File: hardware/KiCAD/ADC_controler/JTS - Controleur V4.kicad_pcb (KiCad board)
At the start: 2 copper layers, 119 x 114 mm, 26 parts, among them J1 Power in, J5 Power out, Q1 Q_NMOS_DGS, Q2 Q_NMOS_DGS, Q3 Q_NMOS_DGS, U1 AD797

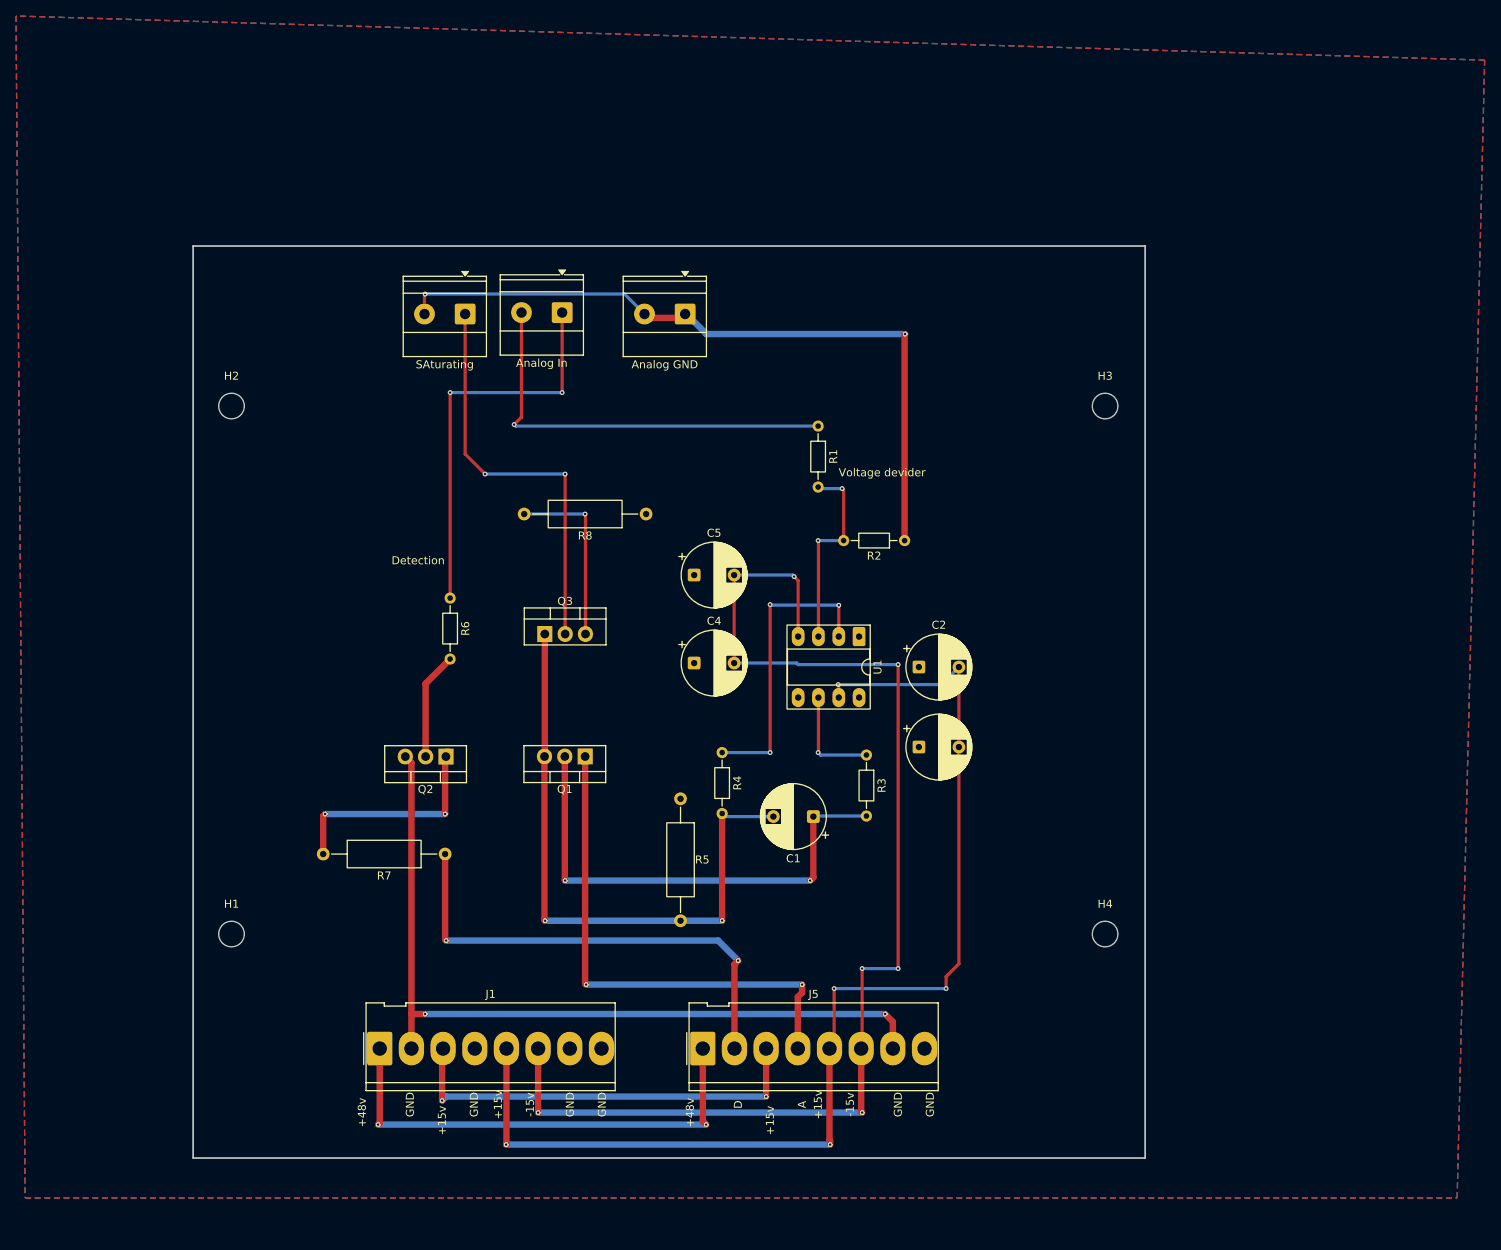
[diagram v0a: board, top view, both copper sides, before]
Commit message: new kicad files
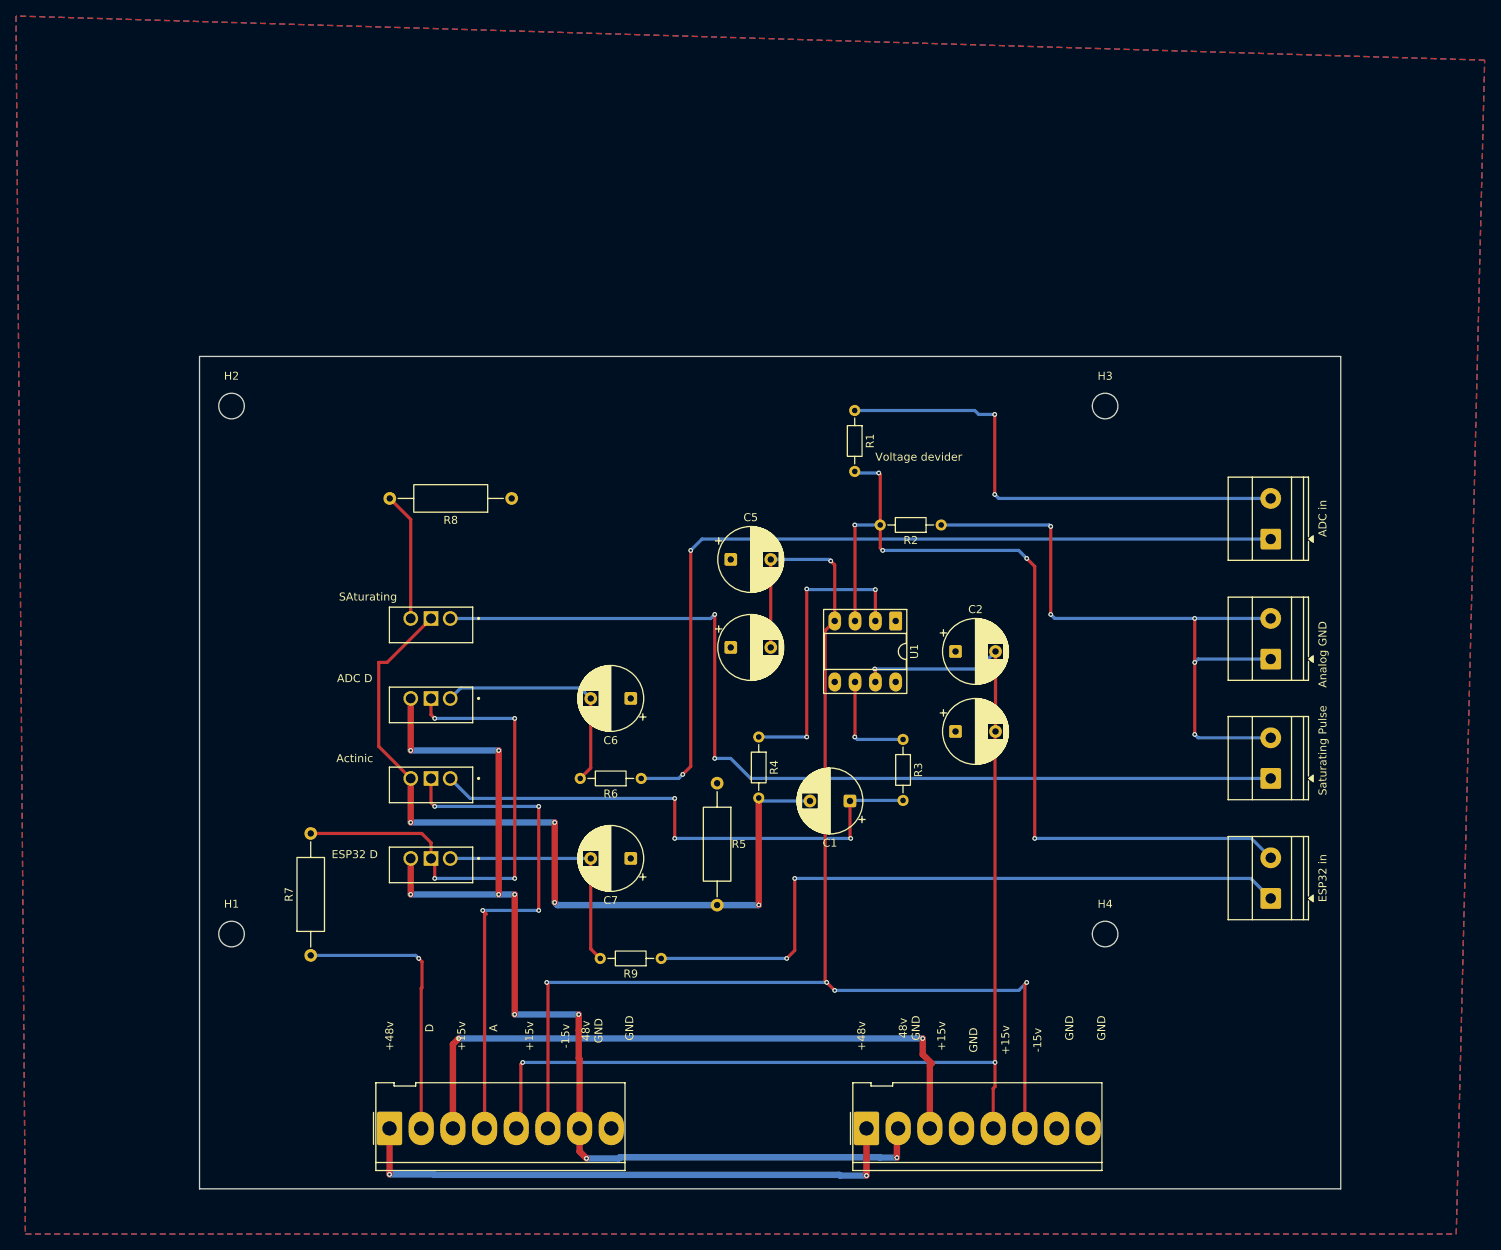
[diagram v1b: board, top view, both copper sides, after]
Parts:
- added C6: C, Capacitor_THT:CP_Radial_D8.0mm_P5.00mm, F.Cu at (170.7, 100.5)
- added C7: C, Capacitor_THT:CP_Radial_D8.0mm_P5.00mm, F.Cu at (170.7, 120.5)
- added J8: ESP32 in, TerminalBlock_Phoenix:TerminalBlock_Phoenix_MKDS-1,5-2-5.08_1x02_P5.08mm_Horizontal, F.Cu at (250.7, 125.5)
- added Q4: ESP32 D, IRF540NPBF:TO254P1054X469X1930-3, F.Cu at (145.7, 121.4)
- added R9: 100, Resistor_THT:R_Axial_DIN0204_L3.6mm_D1.6mm_P7.62mm_Horizontal, F.Cu at (174.5, 133.1)
- J4: renamed from Analog In; value Analog in -> ADC in
- J6: renamed from Analog GND
- Q1: value Q_NMOS_DGS -> Actinic; footprint Package_TO_SOT_THT:TO-220-3_Vertical -> IRF540NPBF:TO254P1054X469X1930-3
- Q2: value Q_NMOS_DGS -> ADC D; footprint Package_TO_SOT_THT:TO-220-3_Vertical -> IRF540NPBF:TO254P1054X469X1930-3
- Q3: value Q_NMOS_DGS -> SAturating; footprint Package_TO_SOT_THT:TO-220-3_Vertical -> IRF540NPBF:TO254P1054X469X1930-3
- R6: value R -> 100
- moved J7 116.2 mm to (250.7, 110.5), turned to 90 degrees
- moved J4 93.0 mm to (250.7, 80.6), turned to 90 degrees
- moved J6 85.0 mm to (250.7, 95.6), turned to 90 degrees
- moved J1 61.7 mm to (200.2, 154.3)
- moved J5 40.4 mm to (140.6, 154.3)
- moved R6 32.8 mm to (172.0, 110.5), turned to 180 degrees
- moved R7 21.0 mm to (130.7, 132.7), turned to 90 degrees
- moved Q1 19.6 mm to (145.7, 111.4)
- moved R8 16.9 mm to (155.8, 75.5)
- moved Q3 14.3 mm to (145.7, 91.4), turned to 180 degrees
- moved Q2 6.72 mm to (145.7, 101.4)
- moved R3 4.97 mm to (204.7, 105.7)
- moved C1 4.97 mm to (198.1, 113.4)
- moved C2 4.97 mm to (211.3, 94.7)
- moved C3 4.97 mm to (211.3, 104.7)
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- renumbered SAturating to J7
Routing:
- net Net-(J8-Pin_2): track 24.9 -> 112.5 mm, vias 2 -> 5
- net Net-(J8-Pin_1): track 0.00 -> 86.6 mm, vias 0 -> 2
- net Net-(J7-Pin_1): track 51.0 -> 121.8 mm
- net Net-(J4-Pin_1): track 50.0 -> 106.9 mm
- net Net-(J1-Pin_2): track 100.7 -> 137.3 mm, vias 2 -> 9
- net Net-(Q2-D): track 27.7 -> 62.9 mm, vias 2 -> 4
- net Net-(Q4-G): track 0.00 -> 30.6 mm
- net Net-(J1-Pin_3): track 53.3 -> 81.5 mm
- net Net-(Q1-S): track 78.5 -> 104.6 mm, vias 2 -> 4
- net Net-(J5-Pin_2): track 59.6 -> 35.1 mm, vias 2 -> 1
- net Net-(Q2-G): track 13.5 -> 29.2 mm
- net Net-(J1-Pin_6): track 156.0 -> 169.7 mm, vias 6 -> 5
- net Net-(J1-Pin_1): track 60.3 -> 72.6 mm
- net Net-(J4-Pin_2): track 52.5 -> 62.4 mm, vias 1 -> 2
- net Net-(Q3-S): track 22.6 -> 16.1 mm, vias 1 -> 0
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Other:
- board size 119 x 114 mm -> 142.6 x 104 mm
- board text added: "48v GND"
- board text removed: "Detection"
